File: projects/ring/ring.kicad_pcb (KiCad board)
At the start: 4 copper layers, 10 x 18 mm, 4 parts, among them U1 STM32WB55CEU6TR, Y1 NX1612SA-32.000MHZ-CHP-CIS-3

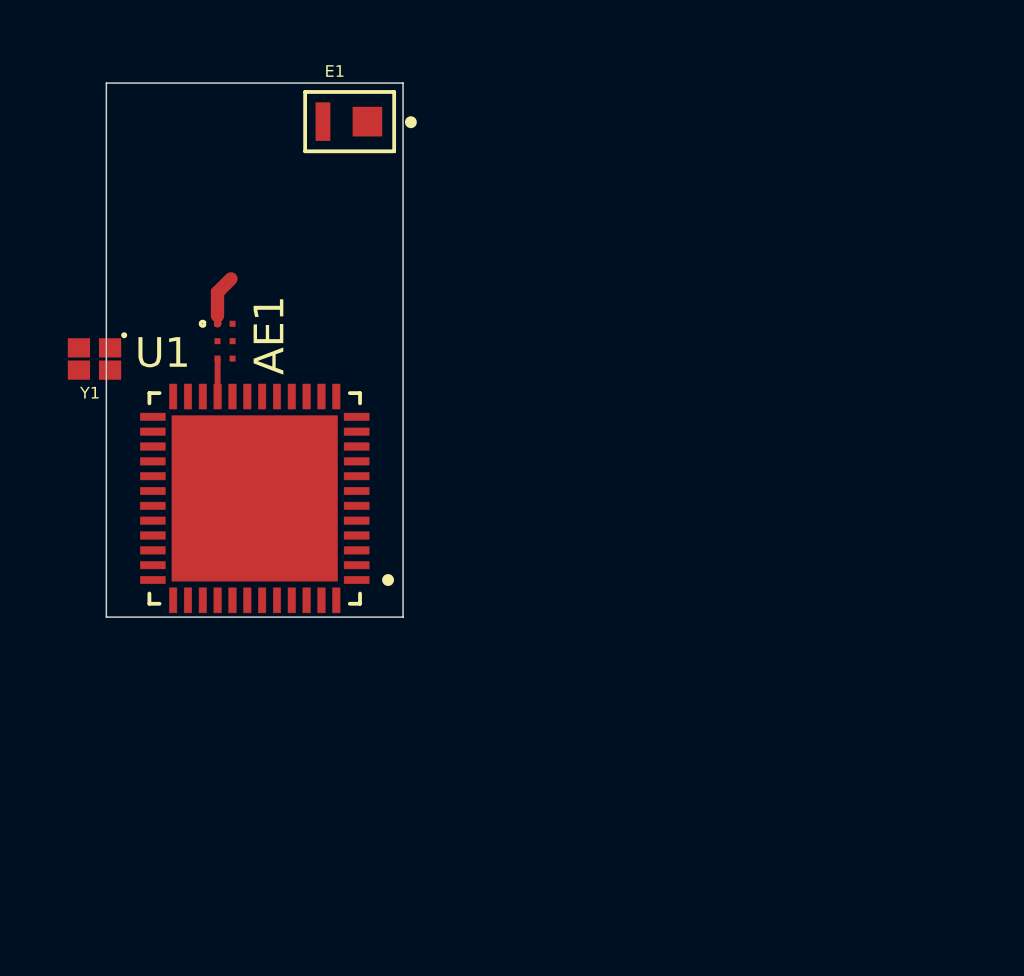
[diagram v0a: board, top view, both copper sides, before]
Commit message: layout and schem changes
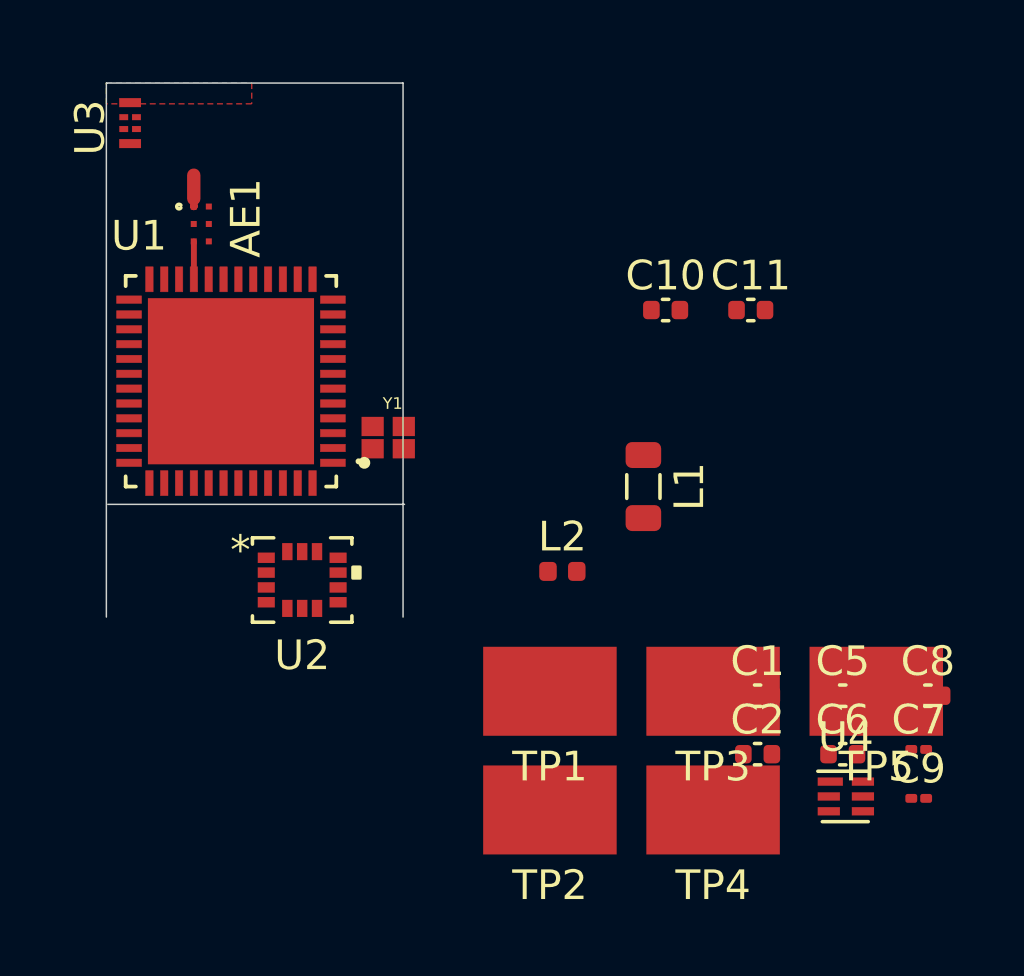
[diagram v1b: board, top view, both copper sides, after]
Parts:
- removed E1: NN02-101, step-footprints:XCVR_NN02-101
- added C1: C_100nF, Capacitor_SMD:C_0402_1005Metric, F.Cu at (91.0, 39.6)
- added C10: C_100nF, Capacitor_SMD:C_0402_1005Metric, F.Cu at (87.8, 26.6)
- added C11: C_100nF, Capacitor_SMD:C_0402_1005Metric, F.Cu at (90.7, 26.6)
- added C2: C_100nF, Capacitor_SMD:C_0402_1005Metric, F.Cu at (91.0, 41.6)
- added C5: C_100nF, Capacitor_SMD:C_0402_1005Metric, F.Cu at (93.8, 39.6)
- added C6: C_100nF, Capacitor_SMD:C_0402_1005Metric, F.Cu at (93.8, 41.6)
- added C7: C_4.7uF, Capacitor_SMD:C_01005_0402Metric, F.Cu at (96.4, 41.5)
- added C8: C_100nF, Capacitor_SMD:C_0402_1005Metric, F.Cu at (96.7, 39.6)
- added C9: C_4.7uF, Capacitor_SMD:C_01005_0402Metric, F.Cu at (96.4, 43.1)
- added L1: L_10uH_LQM21FN100M70L, Inductor_SMD:L_0805_2012Metric, F.Cu at (87.1, 32.6)
- added L2: L_10nH_LQG15WZ10NJ02D, Inductor_SMD:L_0402_1005Metric, F.Cu at (84.4, 35.5)
- added TP1: Test_Point_SMD, footprints:Test_Point_SMD, F.Cu at (84.0, 39.5)
- added TP2: Test_Point_SMD, footprints:Test_Point_SMD, F.Cu at (84.0, 43.5)
- added TP3: Test_Point_SMD, footprints:Test_Point_SMD, F.Cu at (89.5, 39.5)
- added TP4: Test_Point_SMD, footprints:Test_Point_SMD, F.Cu at (89.5, 43.5)
- added TP5: Test_Point_SMD, footprints:Test_Point_SMD, F.Cu at (95.0, 39.5)
- added U2: LSM6DSO32TR, step-footprints:LSM6DSO32TR, F.Cu at (75.6, 35.8)
- added U3: ANT016008LCS2442MA2, step-footprints:ANT016008LCS2442MA2, F.Cu at (69.8, 20.4)
- added U4: BQ297xy, Package_SON:WSON-6_1.5x1.5mm_P0.5mm, F.Cu at (93.9, 43.0)
- moved Y1 10.2 mm to (78.5, 30.9), turned to 0 degrees
- moved AE1 4.03 mm to (72.2, 23.8)
- moved U1 4.03 mm to (73.2, 29.1)
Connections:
- U1 pad 1: Net-(U1-Pad1) -> Net-(C1-Pad1)
- U1 pad 13: Net-(U1-Pad13) -> /CS
- U1 pad 14: Net-(U1-Pad14) -> /SCK
- U1 pad 15: Net-(U1-Pad15) -> /MISO
- U1 pad 16: Net-(U1-Pad16) -> /MOSI
- U1 pad 20: Net-(U1-Pad20) -> Net-(C1-Pad1)
- U1 pad 22: Net-(U1-Pad22) -> GND
- U1 pad 28: Net-(U1-Pad28) -> /LSM_INT1
- U1 pad 29: Net-(U1-Pad29) -> /LSM_INT2
- U1 pad 32: Net-(U1-Pad32) -> GND
- U1 pad 35: Net-(U1-Pad20) -> Net-(C1-Pad1)
- U1 pad 39: Net-(U1-Pad39) -> /SWDIO
- U1 pad 4: Net-(U1-Pad4) -> /BOOT0
- U1 pad 40: Net-(U1-Pad40) -> Net-(C1-Pad1)
- U1 pad 41: Net-(U1-Pad41) -> /SWCLK
- U1 pad 48: Net-(U1-Pad20) -> Net-(C1-Pad1)
- U1 pad 49: Net-(U1-Pad49) -> GND
- U1 pad 8: Net-(U1-Pad8) -> Net-(C1-Pad1)
- Y1 pad 1: Net-(U1-Pad25) -> Net-(U1-Pad2)
- Y1 pad 3: Net-(U1-Pad24) -> Net-(U1-Pad3)
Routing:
- net Net-(AE1-Pad1): track 1.71 -> 1.06 mm
- added copper zone on F.Cu, net /rad_plane
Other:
- outline, holes or cut-outs redrawn
- board text removed: "10mm Metal Keepout"
- board text removed: "5mm gnd plane"
